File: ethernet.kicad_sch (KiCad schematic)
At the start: 45 parts, among them J5 Bus_RJ45_5-2337992-8, Q12 PJE138K, U10 ULS-12/5-D48N-C, U8 TPS2372-3RGWR, U9 ACPL-217-500E

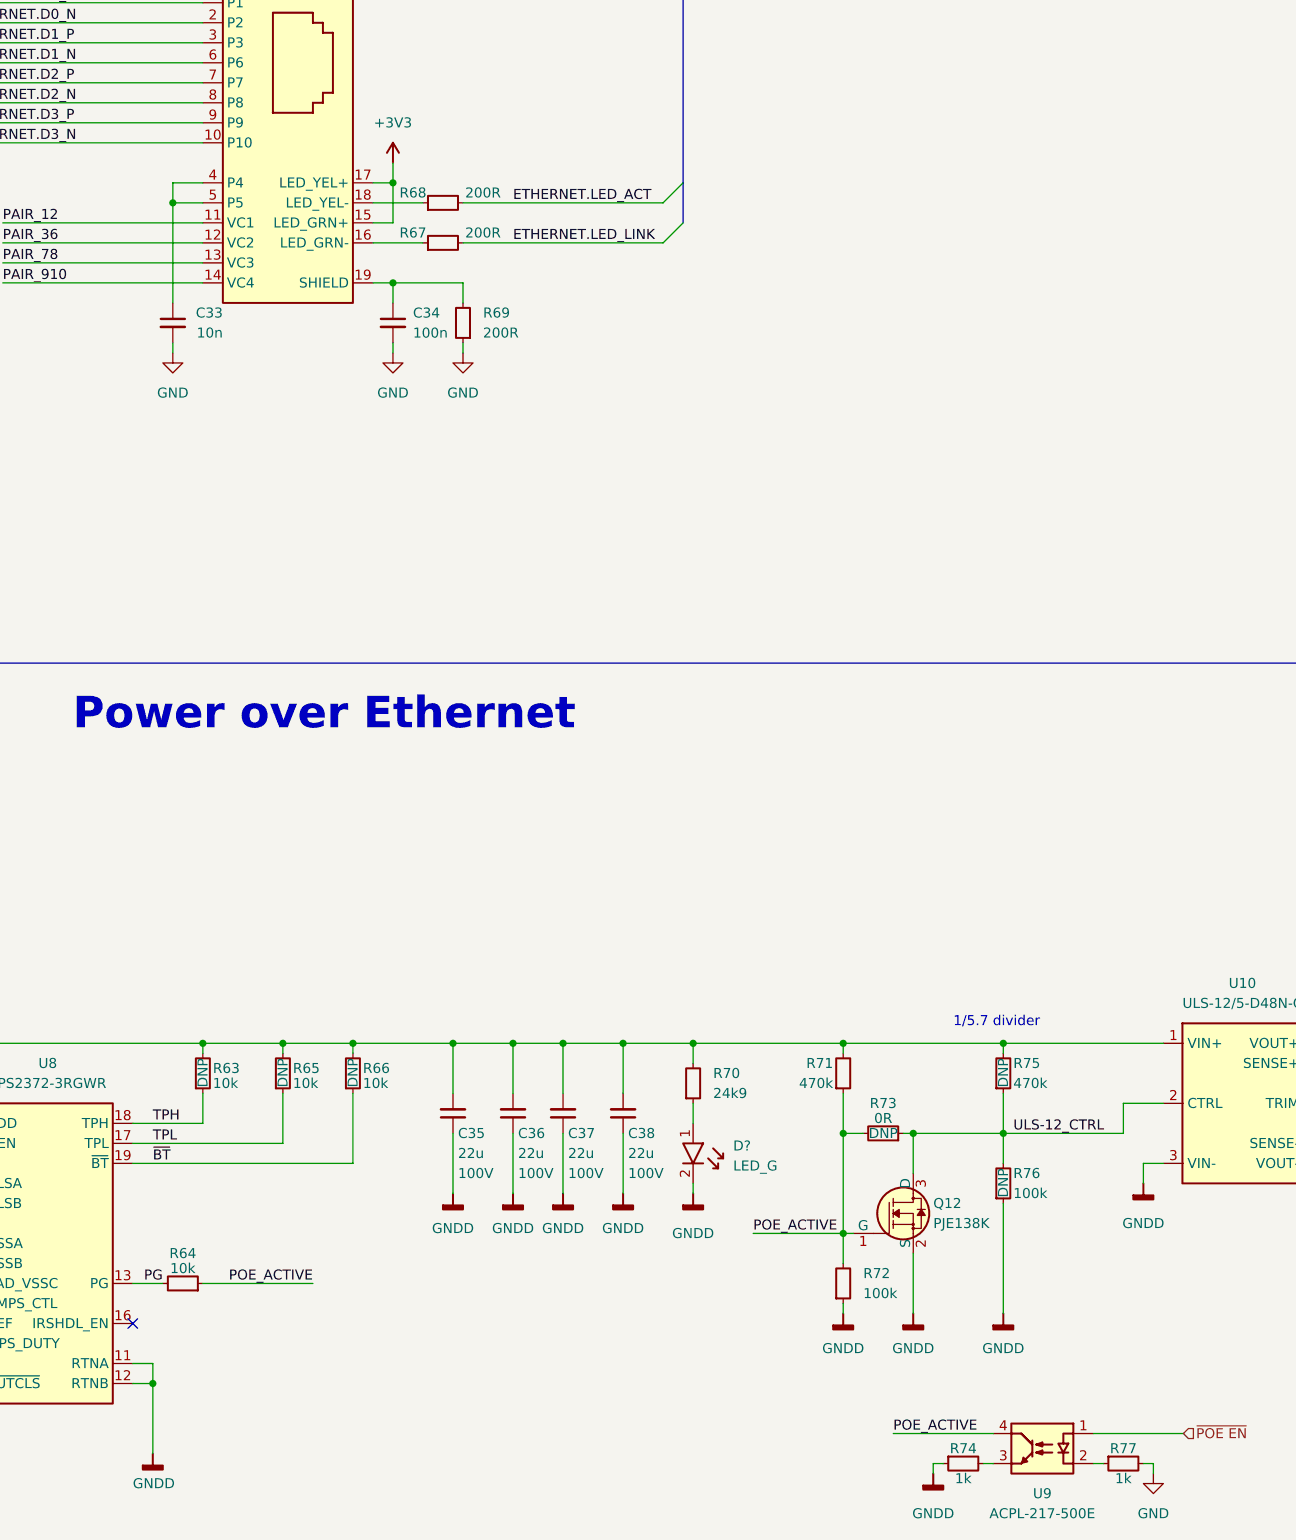
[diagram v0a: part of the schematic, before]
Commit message: [#54617] Review requested changes
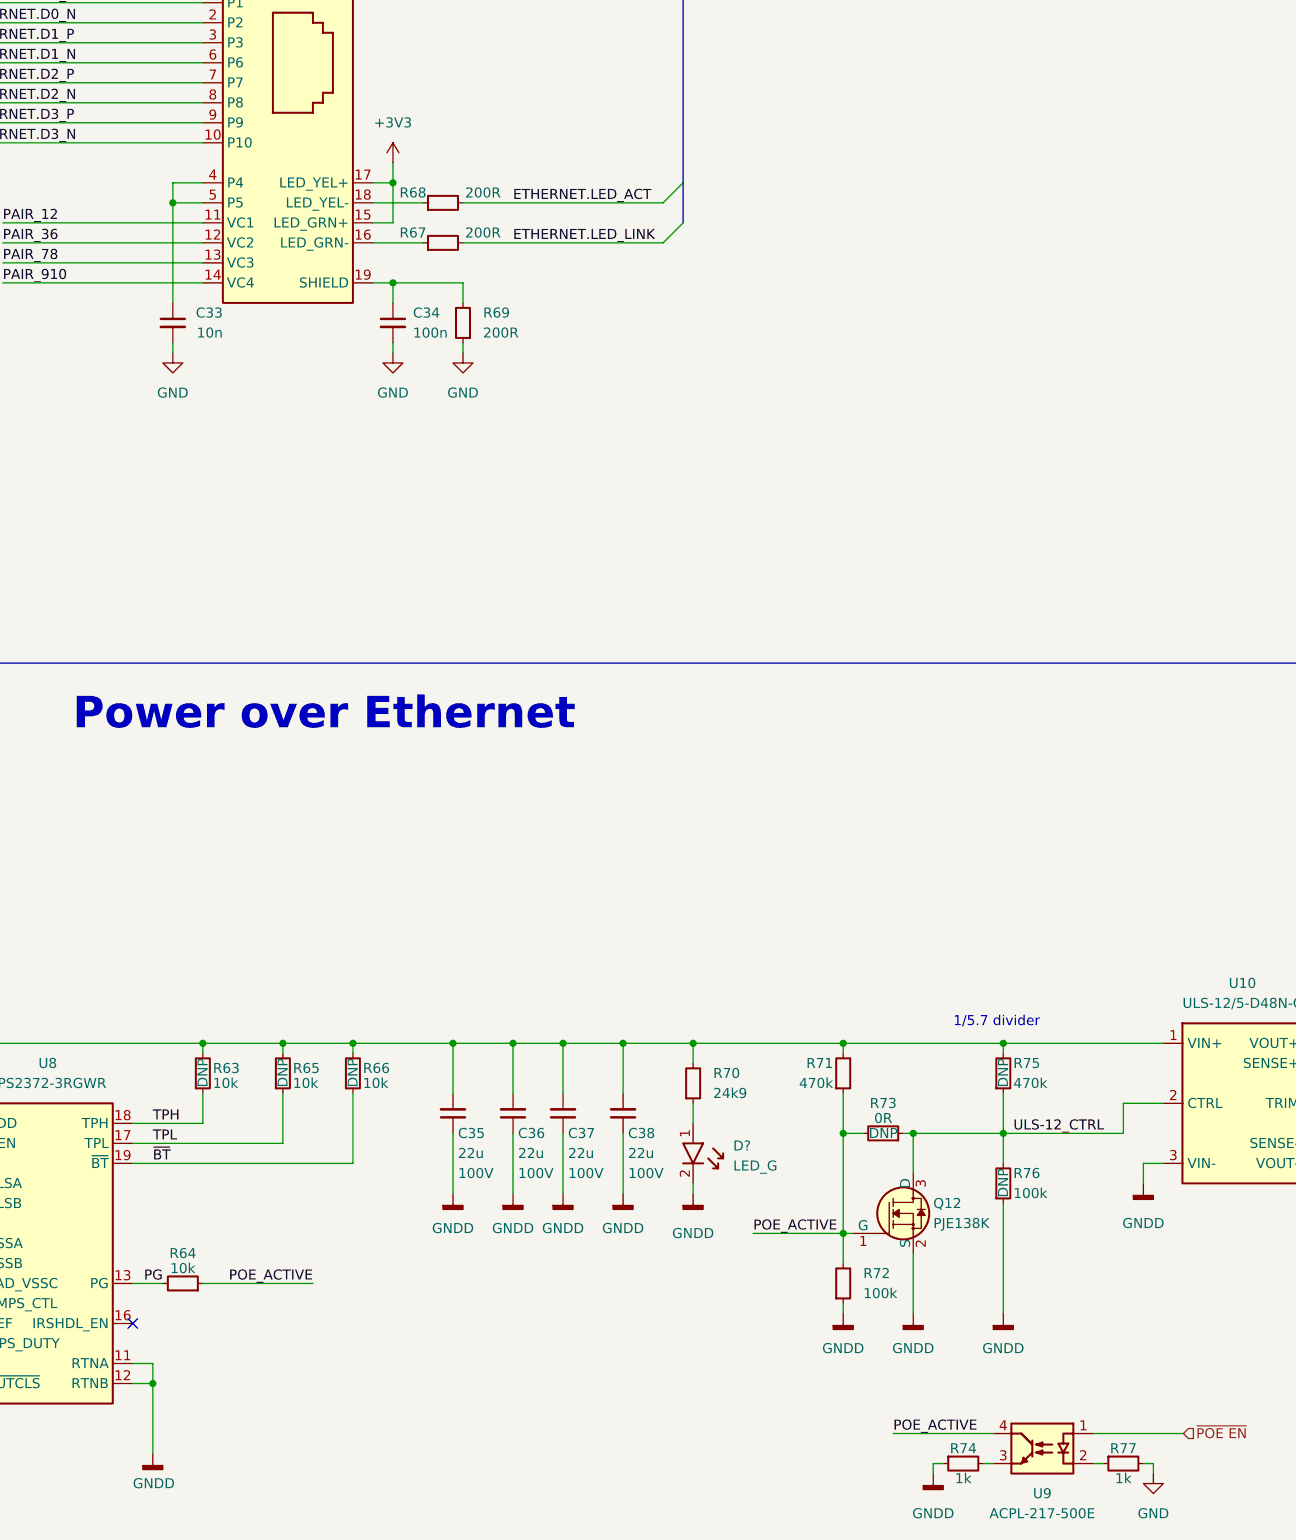
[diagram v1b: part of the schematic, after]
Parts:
- Q12: Manufacturer Panjit -> PANJIT
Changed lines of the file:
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@@
       (effects (font (size 1.27 1.27) (thickness 0.15)) (justify left bottom) hide)
     )
-    (property "Datasheet" "https://search.murata.co.jp/Ceramy/image/img/A01X/G101/ENG/GRM155R61H104KE14-01.pdf" (at 378.46 208.28 0)
+    (property "Datasheet" "https://www.murata.com/products/productdetail?partno=GRM155R61H104KE14%23" (at 378.46 208.28 0)
       (effects (font (size 1.27 1.27) (thickness 0.15)) (justify left bottom) hide)
     )
@@
       (effects (font (size 1.27 1.27) (thickness 0.15)) (justify left bottom) hide)
     )
-    (property "Datasheet" "https://www.mouser.pl/datasheet/2/1057/PJE138K-1876698.pdf" (at 290.83 220.98 0)
+    (property "Datasheet" "https://www.mouser.com/datasheet/2/1057/PJE138K-1876698.pdf" (at 290.83 220.98 0)
       (effects (font (size 1.27 1.27) (thickness 0.15)) (justify left bottom) hide)
     )
@@
       (effects (font (size 1.27 1.27) (thickness 0.15)) (justify left bottom) hide)
     )
-    (property "Manufacturer" "Panjit" (at 290.83 226.06 0)
+    (property "Manufacturer" "PANJIT" (at 290.83 226.06 0)
       (effects (font (size 1.27 1.27) (thickness 0.15)) (justify left bottom) hide)
     )
@@
       (effects (font (size 1.27 1.27) (thickness 0.15)) (justify left bottom) hide)
     )
-    (property "Datasheet" "https://search.murata.co.jp/Ceramy/image/img/A01X/G101/ENG/GRM155R71H103KA88-01.pdf" (at 166.37 109.22 0)
+    (property "Datasheet" "https://www.murata.com/products/productdetail?partno=GRM155R71H103KA88%23" (at 166.37 109.22 0)
       (effects (font (size 1.27 1.27) (thickness 0.15)) (justify left bottom) hide)
     )
@@
       (effects (font (size 1.27 1.27) (thickness 0.15)) (justify left bottom) hide)
     )
-    (property "Datasheet" "https://search.murata.co.jp/Ceramy/image/img/A01X/G101/ENG/GRM155R61H104KE14-01.pdf" (at 224.79 109.22 0)
-      (effects (font (size 1.27 1.27) (thickness 0.15)) (justify left bottom) hide)
-    )
+    (property "Datasheet" "https://www.murata.com/products/productdetail?partno=GRM155R61H104KE14%23" (at 224.79 109.22 0)
+      (effects (font (size 1.27 1.27) (thickness 0.15)) (justify left bottom) hide)
+    )
